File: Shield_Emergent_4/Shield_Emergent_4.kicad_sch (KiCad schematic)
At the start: 29 parts, among them J1 USB3_B_Micro, J2 Conn_01x04_Socket, J3 USB3_B_Micro, J4 Conn_01x05, J5 Conn_01x02_Socket, J6 Conn_01x02_Socket, J7 Conn_01x05, J8 Conn_01x10, U3 SP3012-06UTG, U4 SP3012-06UTG, U5 SP3012-06UTG, U6 SP3012-06UTG, X1 USB_C_24pins

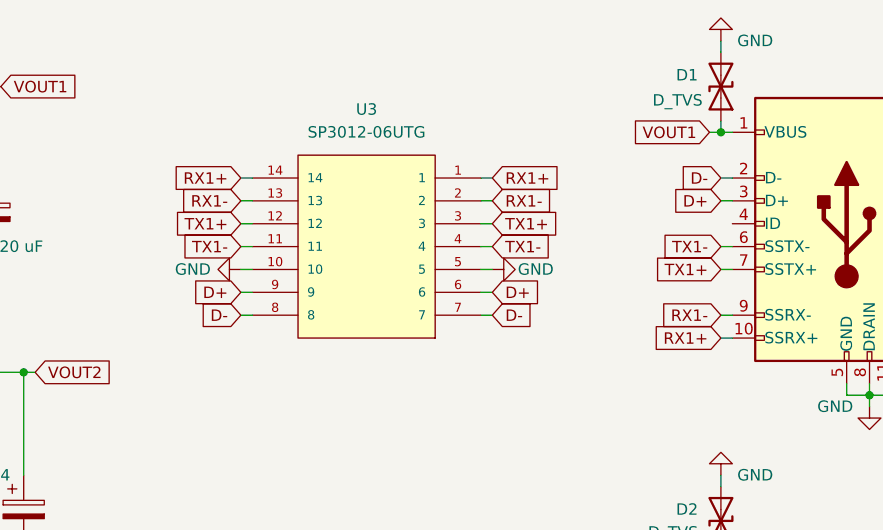
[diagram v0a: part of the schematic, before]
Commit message: v0.5 modified and ordered
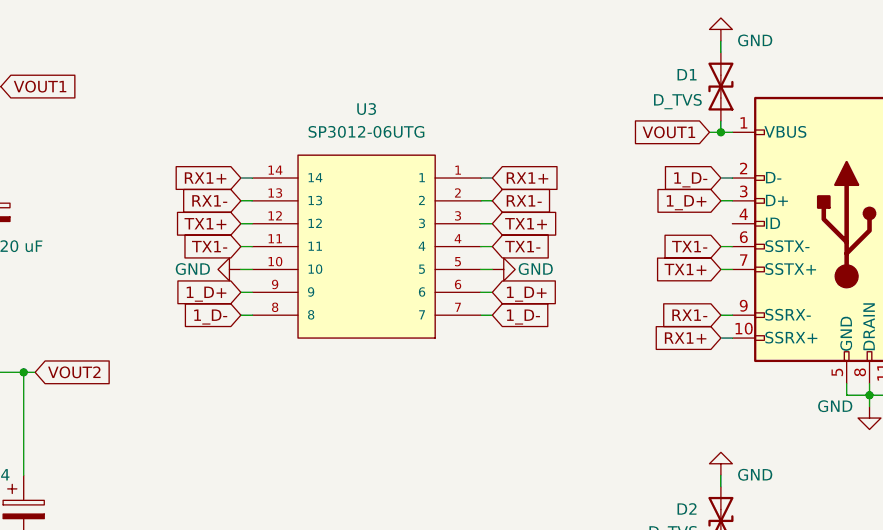
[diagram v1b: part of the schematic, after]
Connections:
- net D+: no longer J1.3 (D+), U3.6, U3.9
- net D-: no longer J1.2 (D-), U3.7, U3.8
- new net 1_D+: J1.3 (D+), U3.6, U3.9
- new net 1_D-: J1.2 (D-), U3.7, U3.8

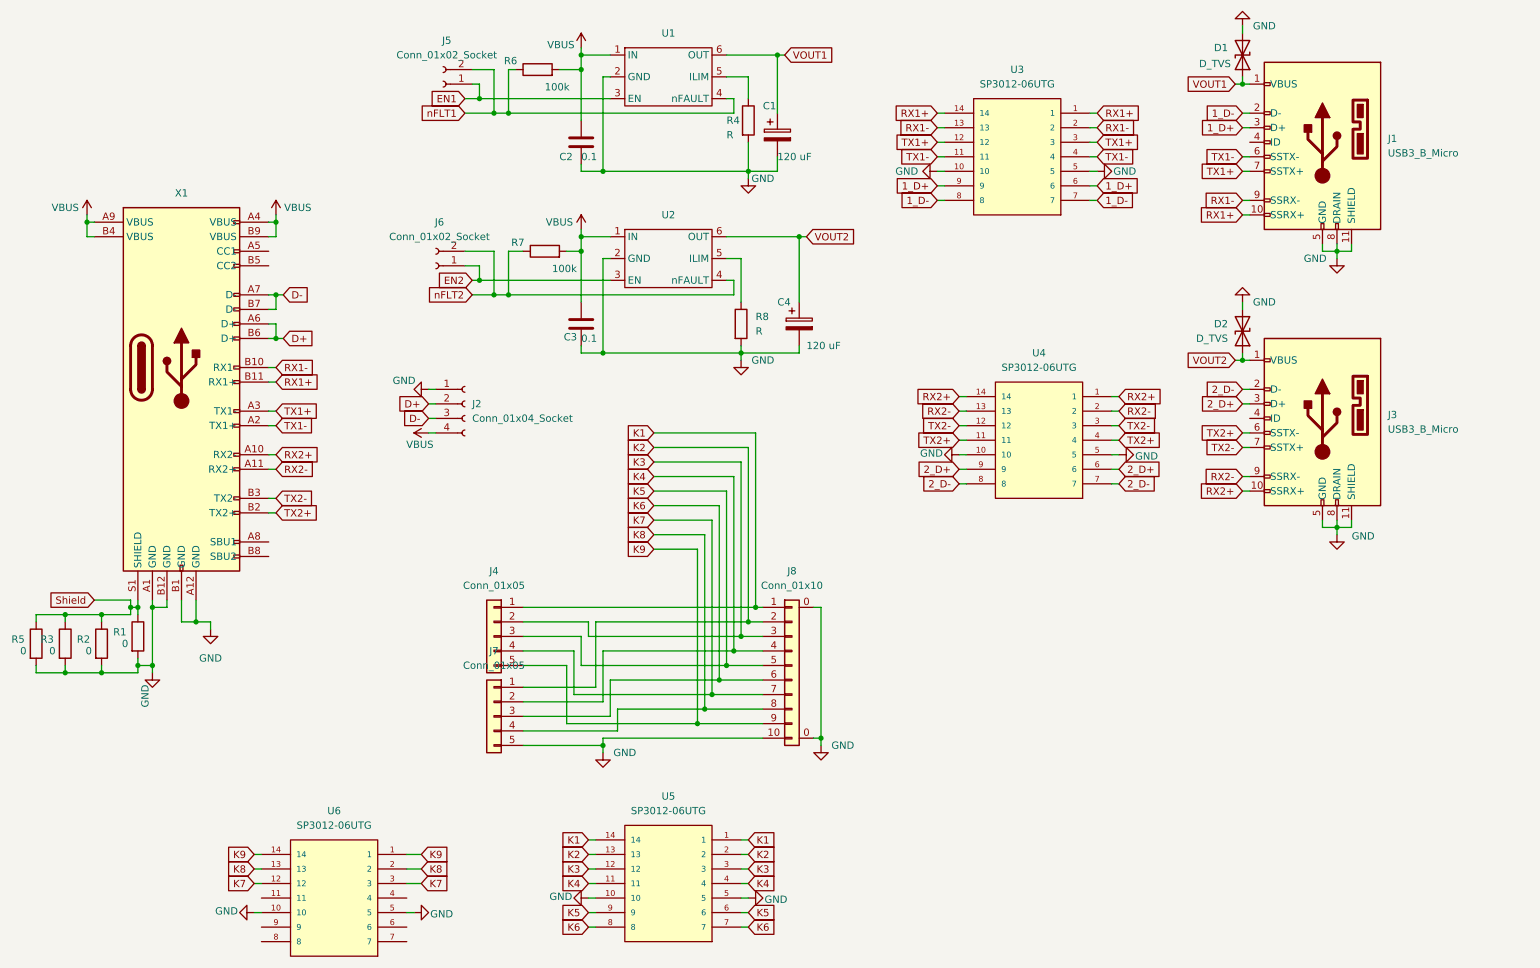
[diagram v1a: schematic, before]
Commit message: v0.6 new geometry
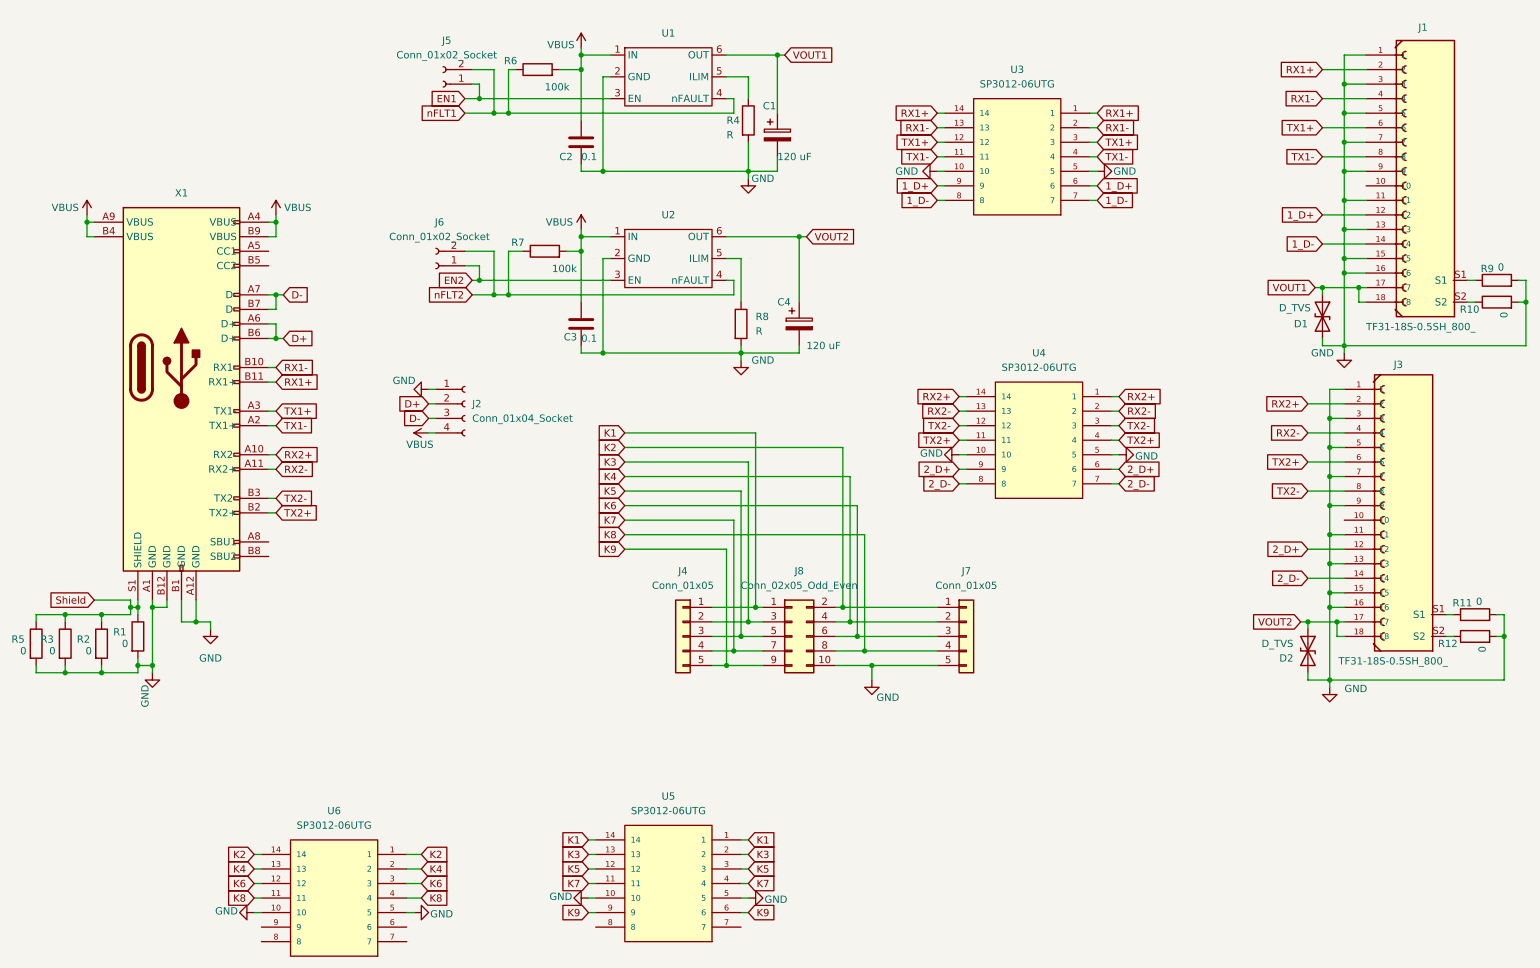
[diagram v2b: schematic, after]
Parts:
- removed J1, J3: USB3_B_Micro, USB_Conns:MU3MS04, symbol Connector:USB3_B_Micro
- removed J8: Conn_01x10, myLib8:50A-10LB, symbol Vedrofara:Conn_01x10
- added J1, J3: TF31-18S-0.5SH_800_, my8lib:HRS_TF31-18S-0.5SH_800_, symbol my8lib:TF31-18S-0.5SH_800_
- added J8: Conn_02x05_Odd_Even, Connector_PinHeader_1.27mm:PinHeader_2x05_P1.27mm_Vertical, symbol Connector_Generic:Conn_02x05_Odd_Even
- added R10, R11, R12, R9: 0, Resistor_SMD:R_0201_0603Metric_Pad0.64x0.40mm_HandSolder, symbol Device:R
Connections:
- net 1_D+: now also J1.12
- net 1_D-: now also J1.14
- net 2_D+: now also J3.12
- net 2_D-: now also J3.14
- net GND: now also J1.1, J1.11, J1.13, J1.15, J1.16, J1.3, J1.5, J1.7, J1.9, J3.1, J3.11, J3.13, J3.15, J3.16, J3.3, J3.5, J3.7, J3.9, J8.10 (Pin_10), R10.2, R11.2, R12.2, R9.2
- net K1: now also J8.1 (Pin_1)
- net K2: now also U6.1, U6.14, J8.2 (Pin_2); no longer U5.13, U5.2
- net K3: now also U5.13, U5.2, J8.3 (Pin_3); no longer U5.12, U5.3
- net K4: now also U6.13, U6.2, J8.4 (Pin_4); no longer U5.11, U5.4
- net K5: now also U5.12, U5.3, J8.5 (Pin_5); no longer U5.6, U5.9
- net K6: now also U6.12, U6.3, J8.6 (Pin_6); no longer U5.7, U5.8
- net K7: now also U5.11, U5.4, J8.7 (Pin_7); no longer U6.12, U6.3
- net K8: now also U6.11, U6.4, J8.8 (Pin_8); no longer U6.13, U6.2
- net K9: now also U5.6, U5.9, J8.9 (Pin_9); no longer U6.1, U6.14
- net RX1+: now also J1.2
- net RX1-: now also J1.4
- net RX2+: now also J3.2
- net RX2-: now also J3.4
- net TX1+: now also J1.6
- net TX1-: now also J1.8
- net TX2+: now also J3.6
- net TX2-: now also J3.8
- net VOUT1: now also J1.17, J1.18
- net VOUT2: now also J3.17, J3.18
- new net: J1.S1, R9.1
- new net: J1.S2, R10.1
- new net: J3.S1, R11.1
- new net: J3.S2, R12.1
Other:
- moved on the sheet: D1, D2, J4, J7
